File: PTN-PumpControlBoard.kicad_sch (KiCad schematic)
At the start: 3 parts, among them J1 PUMP, J2 TEMP, J4 FLOW

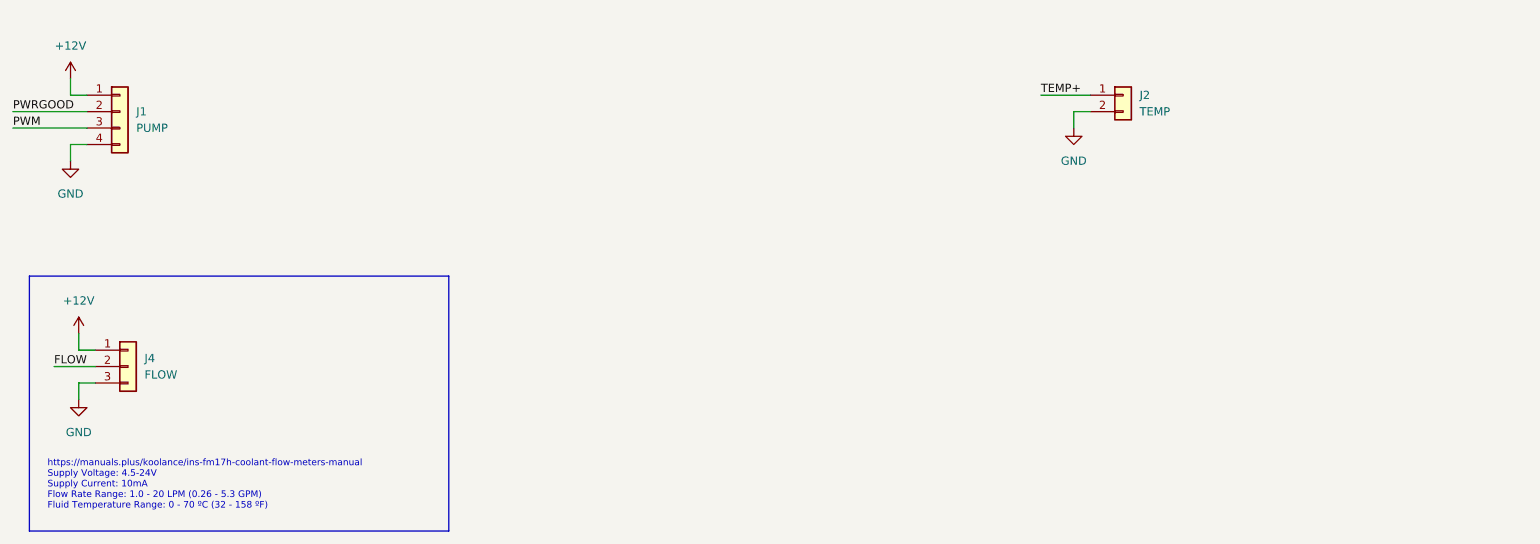
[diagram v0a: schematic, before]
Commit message: testing
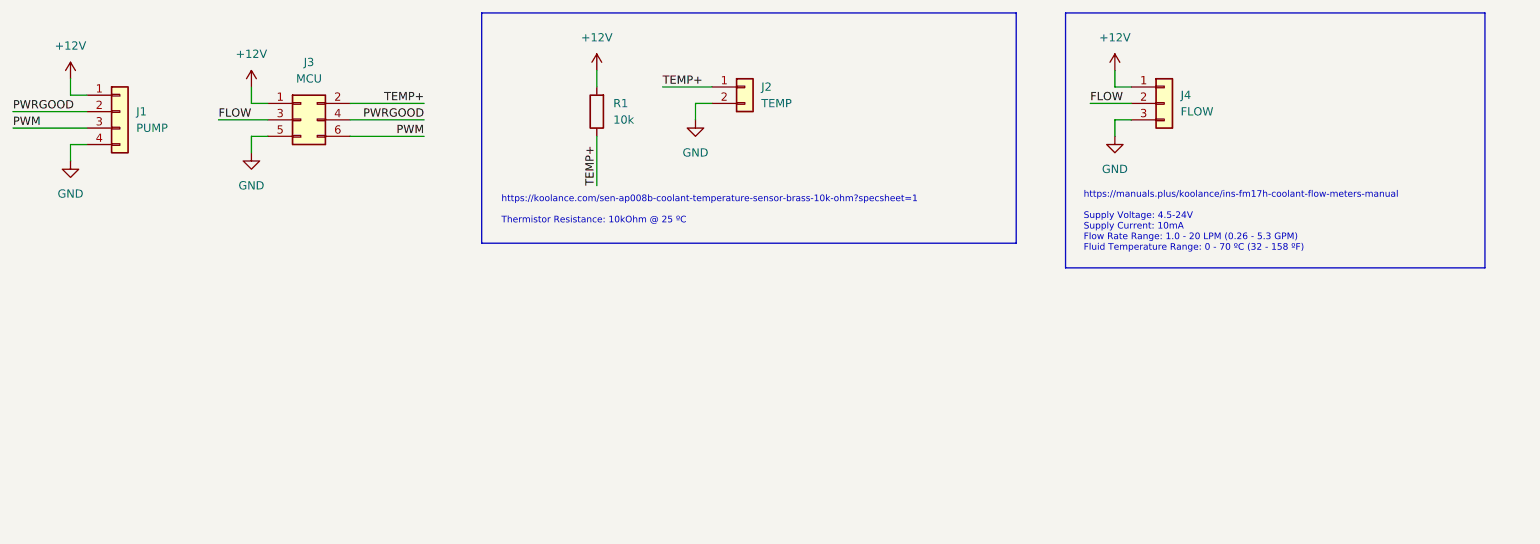
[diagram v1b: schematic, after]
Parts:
- added J3: MCU, symbol Connector_Generic:Conn_02x03_Odd_Even
- added R1: 10k, symbol Device:R
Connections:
- net +12V: now also J3.1 (Pin_1), R1.2
- net FLOW: now also J3.3 (Pin_3)
- net GND: now also J3.5 (Pin_5)
- net PWM: now also J3.6 (Pin_6)
- net PWRGOOD: now also J3.4 (Pin_4)
- net TEMP+: now also J3.2 (Pin_2), R1.1
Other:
- note added: "https://koolance.com/sen-ap008b-coolant-temperature-sensor-brass-10k-ohm?specsheet=1 Thermistor Resistance: 10kOhm @ 25 ºC"
- moved on the sheet: J2, J4
